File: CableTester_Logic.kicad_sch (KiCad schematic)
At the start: 23 parts, among them J1 Power, J10 Conn_Coaxial, J11 Conn_Coaxial, J12 Conn_Coaxial, J13 Conn_Coaxial, J14 Conn_Coaxial, J15 Conn_Coaxial, J16 Conn_Coaxial, J17 Conn_Coaxial, J18 Conn_Coaxial, J19 Conn_Coaxial, J2 PWM, J20 MircoMatch -8, J21 MircoMatch -8, J3 Analog, J4 PWM, J5 Analog, J6 Communication, J7 Digital, J8 Conn_Coaxial, J9 Conn_Coaxial, U1 DG1206EUI+, U2 DG1206EUI+

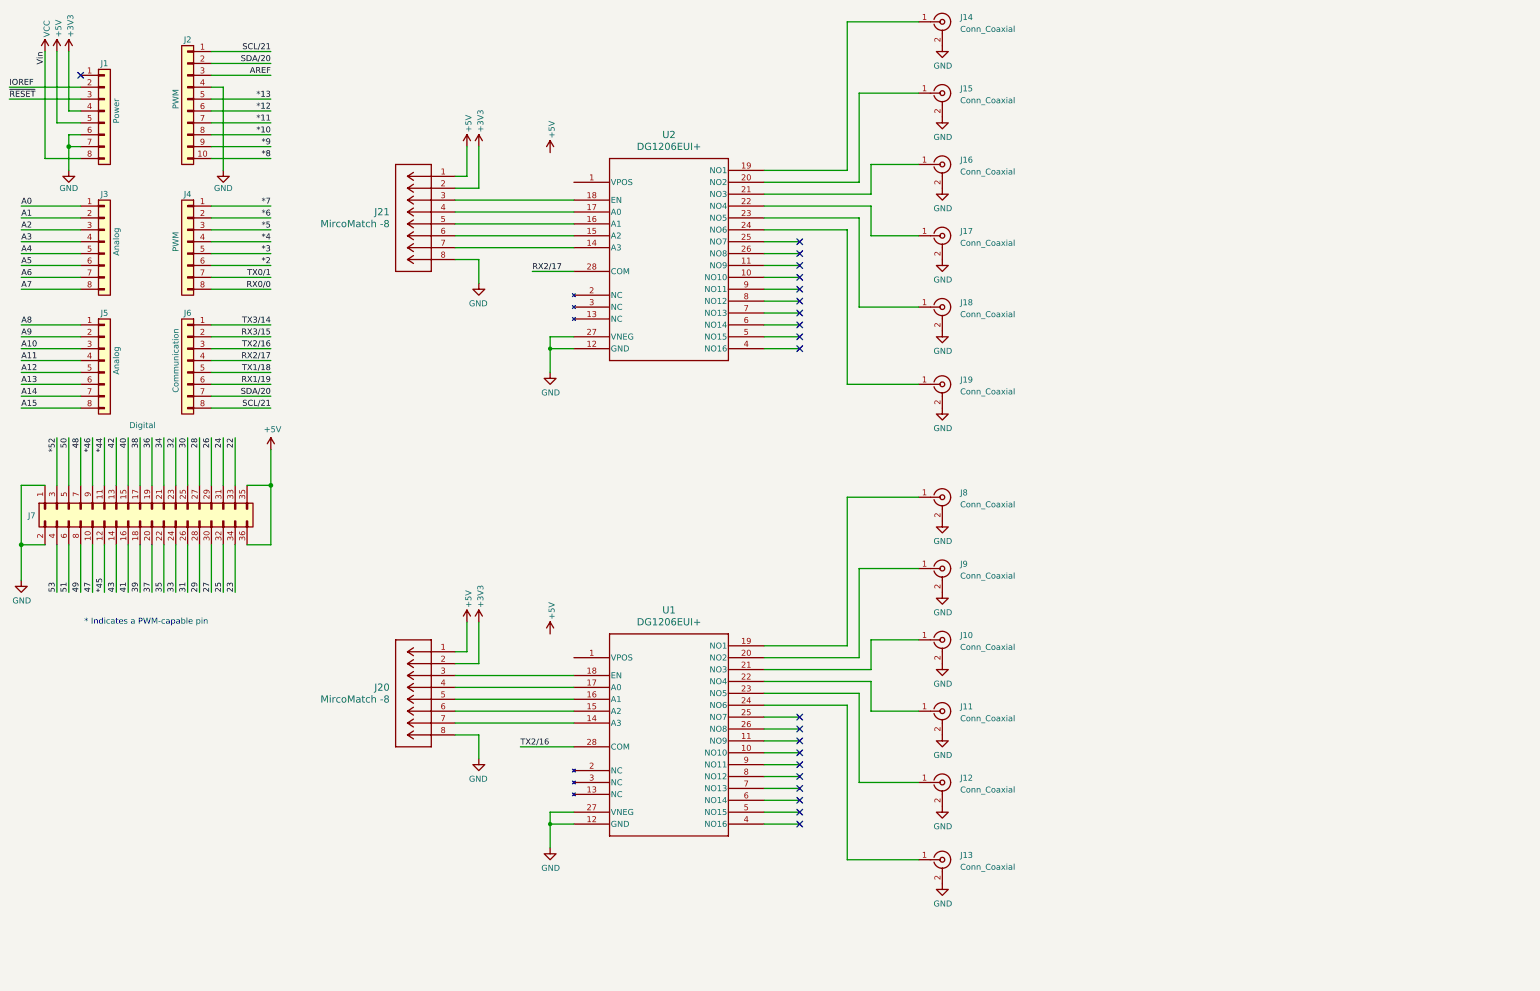
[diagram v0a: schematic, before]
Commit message: Finalized Project for Test Production
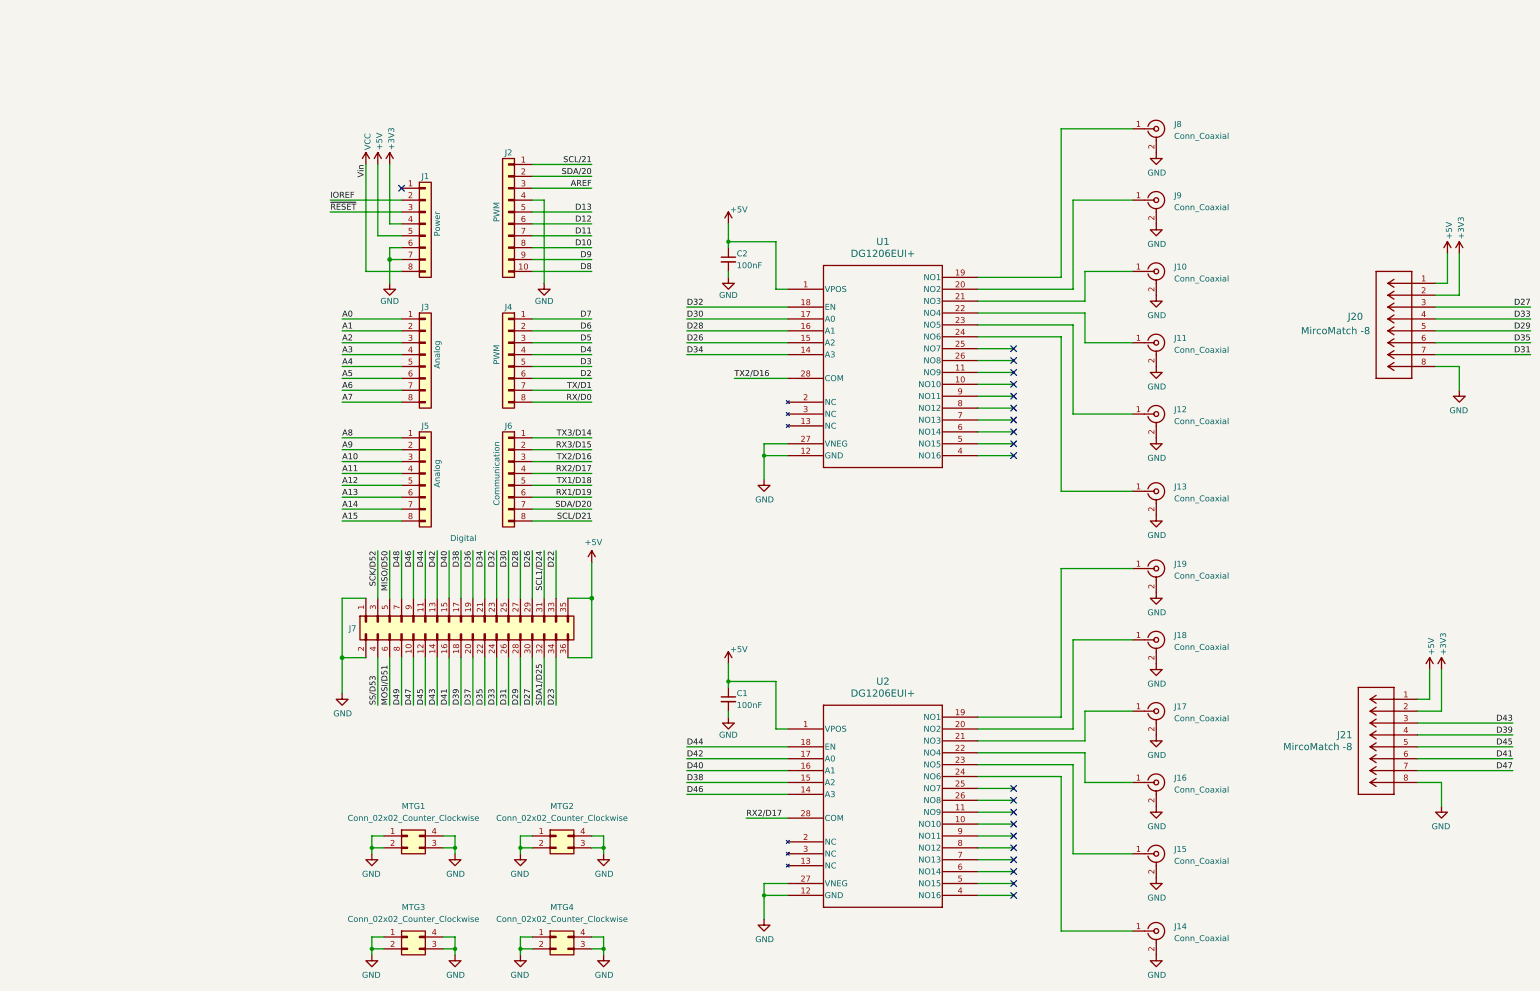
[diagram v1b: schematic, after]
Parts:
- added C1, C2: 100nF, Capacitor_SMD:C_0805_2012Metric_Pad1.18x1.45mm_HandSolder, symbol Device:C_Small
- added MTG1, MTG2, MTG3, MTG4: Conn_02x02_Counter_Clockwise, Project_Footprints:KEYSTONE_7693-5, symbol Connector_Generic:Conn_02x02_Counter_Clockwise
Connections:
- net *46 is gone; now on net D46: J7.9 (Pin_9)
- net 26 is gone; now on net D26: J7.29 (Pin_29)
- net 27 is gone; now on net D27: J7.30 (Pin_30)
- net 28 is gone; now on net D28: J7.27 (Pin_27)
- net 30 is gone; now on net D30: J7.25 (Pin_25)
- net 31 is gone; now on net D31: J7.26 (Pin_26)
- net 38 is gone; now on net D38: J7.17 (Pin_17)
- net 39 is gone; now on net D39: J7.18 (Pin_18)
- net 40 is gone; now on net D40: J7.15 (Pin_15)
- net 43 is gone; now on net D43: J7.14 (Pin_14)
- net +5V: now also U1.1 (VPOS), U2.1 (VPOS), C1.1, C2.1
- net GND: now also C1.2, C2.2, MTG1.1 (Pin_1), MTG1.2 (Pin_2), MTG1.3 (Pin_3), MTG1.4 (Pin_4), MTG2.1 (Pin_1), MTG2.2 (Pin_2), MTG2.3 (Pin_3), MTG2.4 (Pin_4), MTG3.1 (Pin_1), MTG3.2 (Pin_2), MTG3.3 (Pin_3), MTG3.4 (Pin_4), MTG4.1 (Pin_1), MTG4.2 (Pin_2), MTG4.3 (Pin_3), MTG4.4 (Pin_4)
- net SCL/21: no longer J6.8 (Pin_8)
- net SDA/20: no longer J6.7 (Pin_7)
- net D46: now reaches U2.14 (A3)
- net D46: no longer J21.7
- net D38: now reaches U2.15 (A2)
- net D38: no longer J21.6
- net D40: now reaches U2.16 (A1)
- net D40: no longer J21.5
- net D39: now reaches J21.4
- net D39: no longer U2.17 (A0)
- net D43: now reaches J21.3
- net D43: no longer U2.18 (EN)
- net at U2.19 (NO1): now also J19.1 (In); no longer J14.1 (In)
- net at U2.20 (NO2): now also J18.1 (In); no longer J15.1 (In)
- net at U2.21 (NO3): now also J17.1 (In); no longer J16.1 (In)
- net at U2.22 (NO4): now also J16.1 (In); no longer J17.1 (In)
- net at U2.23 (NO5): now also J15.1 (In); no longer J18.1 (In)
- net at U2.24 (NO6): now also J14.1 (In); no longer J19.1 (In)
- net D27: now reaches J20.3
- net D27: no longer U1.18 (EN)
- net D30: now reaches U1.17 (A0)
- net D30: no longer J20.4
- net D28: now reaches U1.16 (A1)
- net D28: no longer J20.5
- net D26: now reaches U1.15 (A2)
- net D26: no longer J20.6
- net D31: now reaches J20.7
- net D31: no longer U1.14 (A3)
- net *10 renamed D10
- net *11 renamed D11
- net *12 renamed D12
- net *13 renamed D13
- net *2 renamed D2
- net *3 renamed D3
- net *4 renamed D4
- net *44 renamed D44
- net D44: now also U2.18 (EN)
- net *45 renamed D45
- net D45: now also J21.5
- net *5 renamed D5
- net *52 renamed SCK/D52
- net *6 renamed D6
- net *7 renamed D7
- net *8 renamed D8
- net *9 renamed D9
- net 22 renamed D22
- net 23 renamed D23
- net 24 renamed SCL1/D24
- net 25 renamed SDA1/D25
- net 29 renamed D29
- net D29: now also J20.5
- net 32 renamed D32
- net D32: now also U1.18 (EN)
- net 33 renamed D33
- net D33: now also J20.4
- net 34 renamed D34
- net D34: now also U1.14 (A3)
- net 35 renamed D35
- net D35: now also J20.6
- net 36 renamed D36
- net 37 renamed D37
- net 41 renamed D41
- net D41: now also J21.6
- net 42 renamed D42
- net D42: now also U2.17 (A0)
- net 47 renamed D47
- net D47: now also J21.7
- net 48 renamed D48
- net 49 renamed D49
- net 50 renamed MISO/D50
- net 51 renamed MOSI/D51
- net 53 renamed SS/D53
- net RX0/0 renamed RX/D0
- net RX1/19 renamed RX1/D19
- net RX2/17 renamed RX2/D17
- net RX3/15 renamed RX3/D15
- net TX0/1 renamed TX/D1
- net TX1/18 renamed TX1/D18
- net TX2/16 renamed TX2/D16
- net TX3/14 renamed TX3/D14
- new net SCL/D21: J6.8 (Pin_8)
- new net SDA/D20: J6.7 (Pin_7)
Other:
- note removed: "* Indicates a PWM-capable pin"
- moved on the sheet: J1, J10, J11, J12, J13, J14, J15, J16, J17, J18, J19, J2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
